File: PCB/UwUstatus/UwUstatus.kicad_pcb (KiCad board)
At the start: 2 copper layers, 26 x 30 mm, 10 parts, among them J1 Conn_01x15, J2 Conn_01x02, J3 Conn_01x06, U2 L7805

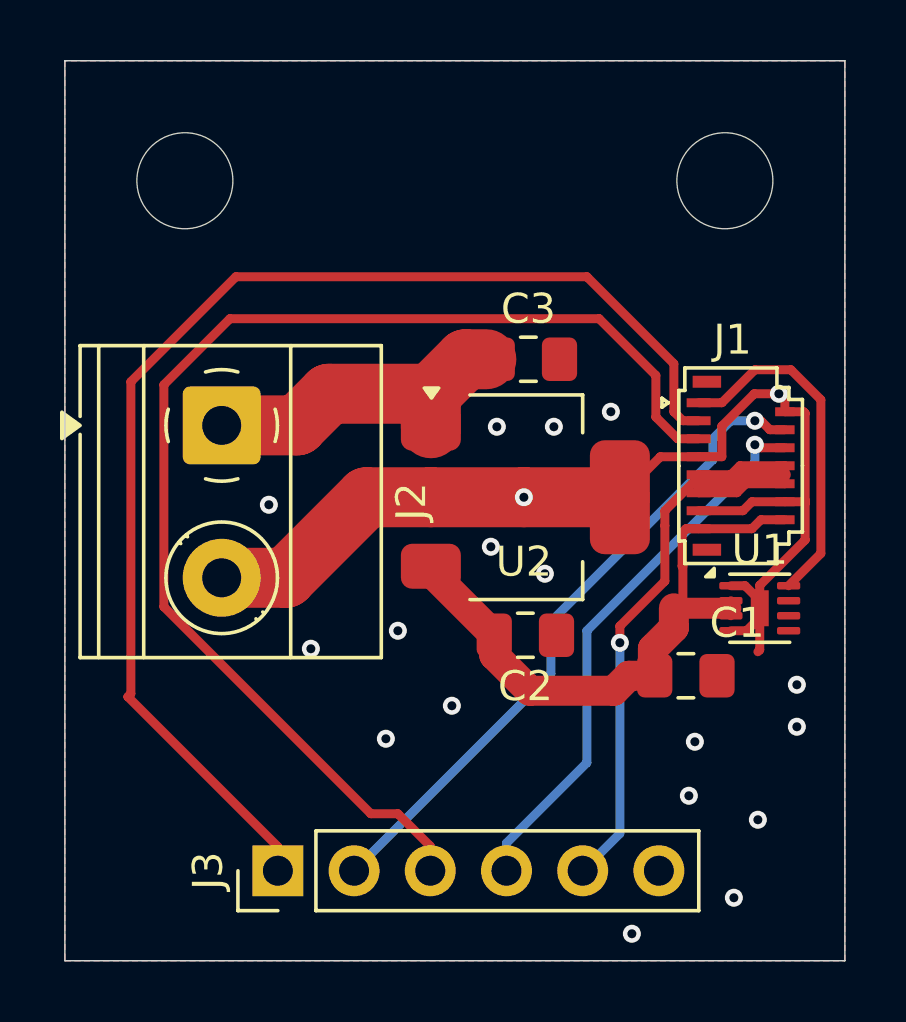
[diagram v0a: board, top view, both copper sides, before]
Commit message: Final revision
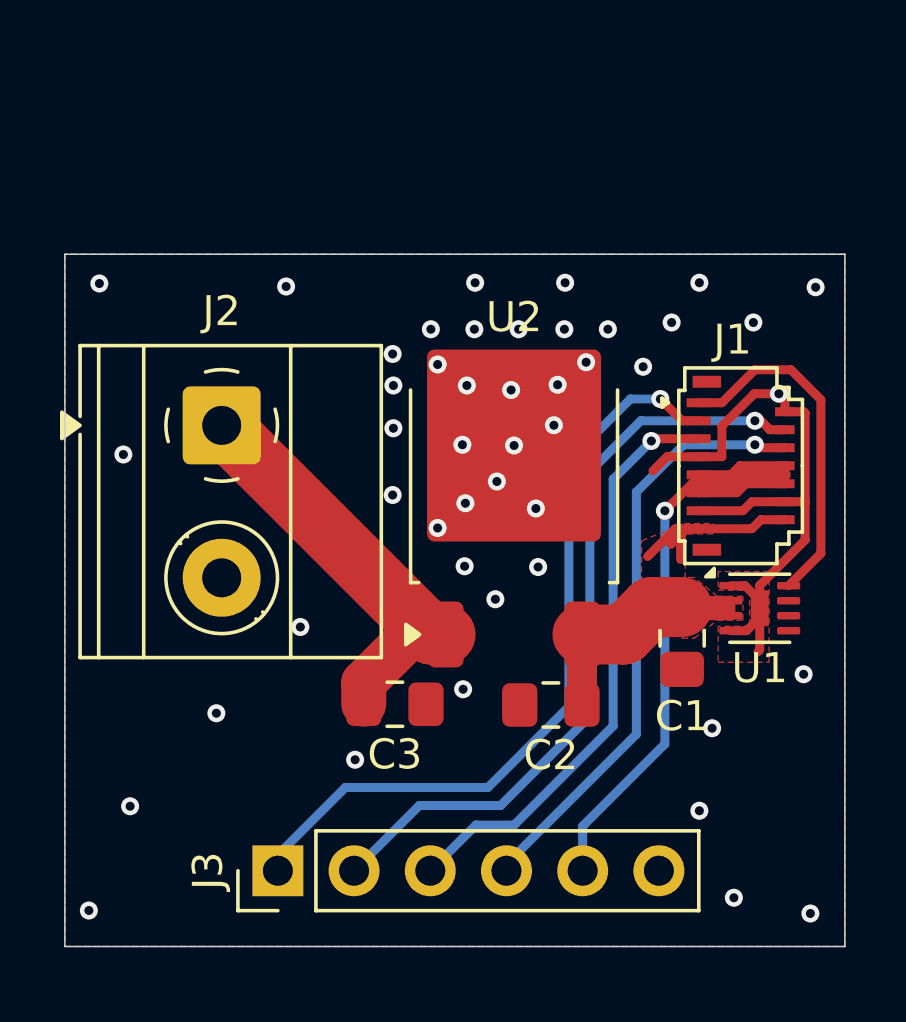
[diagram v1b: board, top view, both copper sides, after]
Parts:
- removed REF** (x2): MountingHole_3.2mm_M3, MountingHole:MountingHole_3.2mm_M3
- added G***: LOGO, d:leeks, B.Cu at (130.1, 64.3)
- U2: footprint Package_TO_SOT_SMD:SOT-223-3_TabPin2 -> Package_TO_SOT_SMD:TO-252-2
- moved C3 12.3 mm to (127.8, 68.0)
- moved C2 2.48 mm to (133.0, 68.0), turned to 180 degrees
- moved C1 1.26 mm to (137.4, 65.8), turned to -90 degrees
- moved U2 0.60 mm to (131.8, 60.6), turned to 90 degrees
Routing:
- net A0: track 41.6 -> 19.7 mm, vias 0 -> 1
- net GND: track 38.9 -> 22.4 mm, vias 19 -> 46
- net FMARK: track 41.7 -> 25.9 mm, vias 0 -> 1
- net SDA: track 22.1 -> 25.5 mm
- net +12V: track 10.9 -> 14.0 mm
- net SCLK: track 18.7 -> 20.1 mm
- net +5V: track 21.1 -> 19.9 mm
- added copper zone on F.Cu, net +5V
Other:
- board size 26 x 30 mm -> 26 x 23.1 mm
